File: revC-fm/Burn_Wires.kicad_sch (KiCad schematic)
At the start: 16 parts, among them J6 T1M-04-F-SV-L, K1 PE014006, Q29 MMDT5551-7-F, Q38 BSZ180P03NS3GATMA1, Q39 MMBT2222LT1G, Q41 BSZ180P03NS3GATMA1

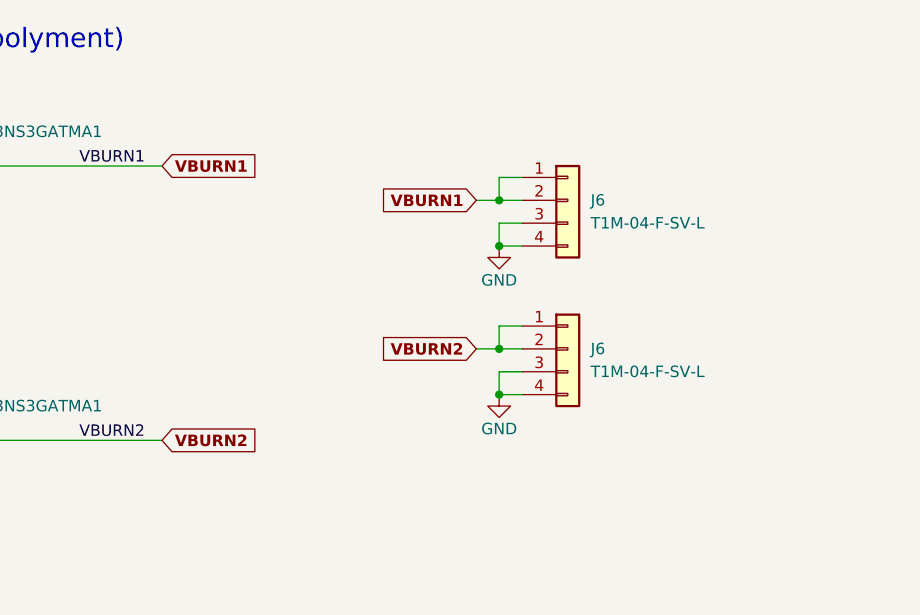
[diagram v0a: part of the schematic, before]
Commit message: routing fm
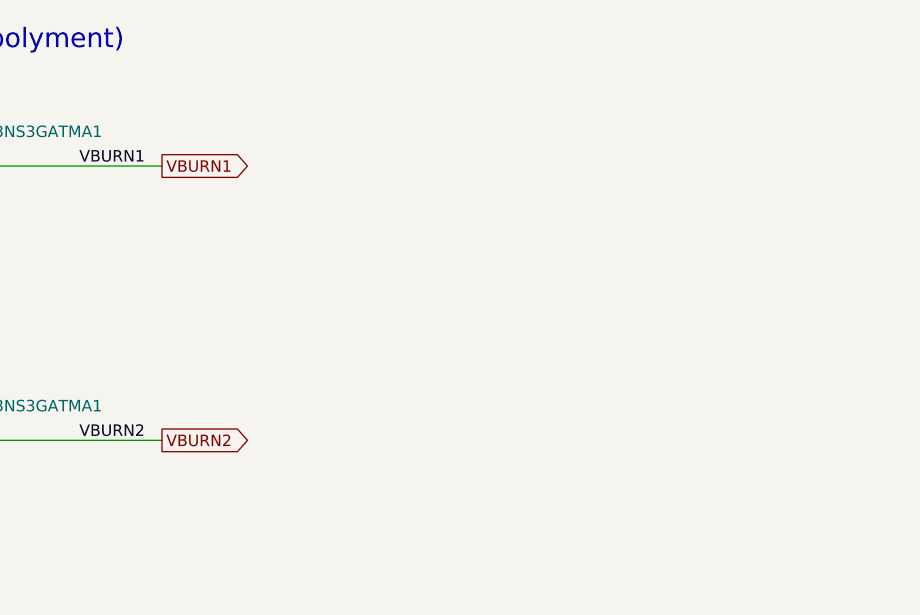
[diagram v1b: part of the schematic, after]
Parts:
- removed J6 (x2): T1M-04-F-SV-L, SierraLobo:SAMTEC_T1M-04-F-SV-L, symbol Connector_Generic:Conn_01x04
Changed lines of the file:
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@@
     (company "Sierra Lobo INC.")
   )
-  (junction (at 252.73 39.37) (diameter 0) (color 0 0 0 0)
-  )
   (junction (at 124.46 30.48) (diameter 0) (color 0 0 0 0)
   )
@@
   (junction (at 58.42 38.1) (diameter 0) (color 0 0 0 0)
   )
-  (junction (at 252.73 50.8) (diameter 0) (color 0 0 0 0)
-  )
   (junction (at 58.42 30.48) (diameter 0) (color 0 0 0 0)
   )
@@
   (junction (at 170.18 60.96) (diameter 0) (color 0 0 0 0)
   )
-  (junction (at 252.73 34.29) (diameter 0) (color 0 0 0 0)
-  )
-  (junction (at 252.73 55.88) (diameter 0) (color 0 0 0 0)
-  )
-  (wire (pts (xy 252.73 36.83) (xy 255.27 36.83))
-    (stroke (width 0) (type default))
-  )
   (wire (pts (xy 170.18 30.48) (xy 170.18 31.75))
     (stroke (width 0) (type default))
@@
     (stroke (width 0) (type default))
   )
-  (wire (pts (xy 252.73 50.8) (xy 255.27 50.8))
-    (stroke (width 0) (type default))
-  )
   (wire (pts (xy 144.78 48.26) (xy 154.94 48.26))
     (stroke (width 0) (type default))
@@
     (stroke (width 0) (type default))
   )
-  (wire (pts (xy 252.73 53.34) (xy 255.27 53.34))
-    (stroke (width 0) (type default))
-  )
   (wire (pts (xy 170.18 60.96) (xy 185.42 60.96))
     (stroke (width 0) (type default))
@@
     (stroke (width 0) (type default))
   )
-  (wire (pts (xy 255.27 31.75) (xy 252.73 31.75))
-    (stroke (width 0) (type default))
-  )
   (wire (pts (xy 170.18 69.85) (xy 170.18 73.025))
     (stroke (width 0) (type default))
@@
     (stroke (width 0) (type default))
   )
-  (wire (pts (xy 252.73 55.88) (xy 252.73 53.34))
-    (stroke (width 0) (type default))
-  )
-  (wire (pts (xy 252.73 31.75) (xy 252.73 34.29))
-    (stroke (width 0) (type default))
-  )
-  (wire (pts (xy 252.73 34.29) (xy 255.27 34.29))
-    (stroke (width 0) (type default))
-  )
   (wire (pts (xy 58.42 52.705) (xy 58.42 55.88))
     (stroke (width 0) (type default))
@@
     (stroke (width 0) (type default))
   )
-  (wire (pts (xy 252.73 39.37) (xy 252.73 36.83))
-    (stroke (width 0) (type default))
-  )
   (wire (pts (xy 124.46 30.48) (xy 170.18 30.48))
     (stroke (width 0) (type default))
   )
-  (wire (pts (xy 250.19 34.29) (xy 252.73 34.29))
-    (stroke (width 0) (type default))
-  )
   (wire (pts (xy 195.58 60.96) (xy 215.265 60.96))
     (stroke (width 0) (type default))
@@
     (stroke (width 0) (type default))
   )
-  (wire (pts (xy 255.27 39.37) (xy 252.73 39.37))
-    (stroke (width 0) (type default))
-  )
   (wire (pts (xy 124.46 60.96) (xy 170.18 60.96))
     (stroke (width 0) (type default))
@@
     (stroke (width 0) (type default))
   )
-  (wire (pts (xy 252.73 48.26) (xy 252.73 50.8))
-    (stroke (width 0) (type default))
-  )
   (wire (pts (xy 38.1 47.625) (xy 41.91 47.625))
     (stroke (width 0) (type default))
@@
     (stroke (width 0) (type default))
   )
-  (wire (pts (xy 250.19 50.8) (xy 252.73 50.8))
-    (stroke (width 0) (type default))
-  )
   (polyline (pts (xy 176.53 162.56) (xy 284.48 162.56))
     (stroke (width 0) (type default))
@@
     (stroke (width 0) (type default))
   )
-  (wire (pts (xy 255.27 48.26) (xy 252.73 48.26))
-    (stroke (width 0) (type default))
-  )
   (wire (pts (xy 58.42 38.1) (xy 63.5 38.1))
     (stroke (width 0) (type default))
   )
   (wire (pts (xy 49.53 47.625) (xy 50.8 47.625))
-    (stroke (width 0) (type default))
-  )
-  (wire (pts (xy 255.27 55.88) (xy 252.73 55.88))
     (stroke (width 0) (type default))
   )
@@
     )
   )
-  (global_label "VBURN1" (shape input) (at 215.265 30.48 0) (fields_autoplaced)
-    (effects (font (size 1.27 1.27) (thickness 0.254) bold) (justify left))
-    (property "Intersheetrefs" "${INTERSHEET_REFS}" (at 1.905 -5.08 0)
-      (effects (font (size 1.27 1.27)) hide)
+  (global_label "VBURN1" (shape output) (at 215.265 30.48 0) (fields_autoplaced)
+    (effects (font (size 1.27 1.27)) (justify left))
+    (property "Intersheetrefs" "${INTERSHEET_REFS}" (at 225.0157 30.48 0)
+      (effects (font (size 1.27 1.27)) (justify left) hide)
     )
   )
@@
     )
   )
-  (global_label "VBURN2" (shape input) (at 250.19 50.8 180) (fields_autoplaced)
-    (effects (font (size 1.27 1.27) (thickness 0.254) bold) (justify right))
-    (property "Intersheetrefs" "${INTERSHEET_REFS}" (at 463.55 -8.89 0)
-      (effects (font (size 1.27 1.27)) (justify left) hide)
-    )
-  )
-  (global_label "VBURN2" (shape input) (at 215.265 60.96 0) (fields_autoplaced)
-    (effects (font (size 1.27 1.27) (thickness 0.254) bold) (justify left))
-    (property "Intersheetrefs" "${INTERSHEET_REFS}" (at 1.905 1.27 0)
-      (effects (font (size 1.27 1.27)) hide)
-    )
-  )
-  (global_label "VBURN1" (shape input) (at 250.19 34.29 180) (fields_autoplaced)
-    (effects (font (size 1.27 1.27) (thickness 0.254) bold) (justify right))
-    (property "Intersheetrefs" "${INTERSHEET_REFS}" (at 463.55 -1.27 0)
+  (global_label "VBURN2" (shape output) (at 215.265 60.96 0) (fields_autoplaced)
+    (effects (font (size 1.27 1.27)) (justify left))
+    (property "Intersheetrefs" "${INTERSHEET_REFS}" (at 225.0157 60.96 0)
       (effects (font (size 1.27 1.27)) (justify left) hide)
     )
@@
     )
   )
-  (symbol (lib_id "power:GND") (at 252.73 39.37 0) (unit 1)
-    (in_bom yes) (on_board yes) (dnp no)
-    (property "Reference" "#PWR0122" (at 252.73 45.72 0)
-      (effects (font (size 1.27 1.27)) hide)
-    )
-    (property "Value" "GND" (at 252.73 43.18 0)
-      (effects (font (size 1.27 1.27)))
-    )
-    (property "Footprint" "" (at 252.73 39.37 0)
-      (effects (font (size 1.27 1.27)) hide)
-    )
-    (property "Datasheet" "" (at 252.73 39.37 0)
-      (effects (font (size 1.27 1.27)) hide)
-    )
-    (pin "1")
-    (instances
-      (project "mainboard"
-        (path "/d1441985-7b63-4bf8-a06d-c70da2e3b78b/00000000-0000-0000-0000-00005cec6476"
-          (reference "#PWR0122") (unit 1)
-        )
-      )
-    )
-  )
   (symbol (lib_id "Transistor_BJT:MMDT5551") (at 167.64 81.28 0) (unit 2)
     (in_bom yes) (on_board yes) (dnp no)
@@
     )
   )
-  (symbol (lib_id "power:GND") (at 252.73 55.88 0) (unit 1)
-    (in_bom yes) (on_board yes) (dnp no)
-    (property "Reference" "#PWR0125" (at 252.73 62.23 0)
-      (effects (font (size 1.27 1.27)) hide)
-    )
-    (property "Value" "GND" (at 252.73 59.69 0)
-      (effects (font (size 1.27 1.27)))
-    )
-    (property "Footprint" "" (at 252.73 55.88 0)
-      (effects (font (size 1.27 1.27)) hide)
-    )
-    (property "Datasheet" "" (at 252.73 55.88 0)
-      (effects (font (size 1.27 1.27)) hide)
-    )
-    (pin "1")
-    (instances
-      (project "mainboard"
-        (path "/d1441985-7b63-4bf8-a06d-c70da2e3b78b/00000000-0000-0000-0000-00005cec6476"
-          (reference "#PWR0125") (unit 1)
-        )
-      )
-    )
-  )
   (symbol (lib_id "Transistor_BJT:MMDT5551") (at 167.64 48.26 0) (unit 2)
     (in_bom yes) (on_board yes) (dnp no)
@@
         )
       )
-    )
-  )
-  (symbol (lib_id "Connector_Generic:Conn_01x04") (at 260.35 50.8 0) (unit 1)
-    (in_bom yes) (on_board yes) (dnp no) (fields_autoplaced)
-    (property "Reference" "J6" (at 262.89 50.7999 0)
-      (effects (font (size 1.27 1.27)) (justify left))
-    )
-    (property "Value" "T1M-04-F-SV-L" (at 262.89 53.3399 0)
-      (effects (font (size 1.27 1.27)) (justify left))
-    )
-    (property "Footprint" "SierraLobo:SAMTEC_T1M-04-F-SV-L" (at 260.35 50.8 0)
-      (effects (font (size 1.27 1.27)) hide)
-    )
-    (property "Datasheet" "~" (at 260.35 50.8 0)
-      (effects (font (size 1.27 1.27)) hide)
-    )
-    (pin "1")
-    (pin "2")
-    (pin "3")
-    (pin "4")
-    (instances
-      (project "mainboard"
-        (path "/d1441985-7b63-4bf8-a06d-c70da2e3b78b/00000000-0000-0000-0000-00005cec60eb"
-          (reference "J6") (unit 1)
-        )
-        (path "/d1441985-7b63-4bf8-a06d-c70da2e3b78b/00000000-0000-0000-0000-00005cec6476"
-          (reference "J5") (unit 1)
-        )
-      )
-    )
-  )
-  (symbol (lib_id "Connector_Generic:Conn_01x04") (at 260.35 34.29 0) (unit 1)
-    (in_bom yes) (on_board yes) (dnp no) (fields_autoplaced)
-    (property "Reference" "J6" (at 262.89 34.2899 0)
-      (effects (font (size 1.27 1.27)) (justify left))
-    )
-    (property "Value" "T1M-04-F-SV-L" (at 262.89 36.8299 0)
-      (effects (font (size 1.27 1.27)) (justify left))
-    )
-    (property "Footprint" "SierraLobo:SAMTEC_T1M-04-F-SV-L" (at 260.35 34.29 0)
-      (effects (font (size 1.27 1.27)) hide)
-    )
-    (property "Datasheet" "~" (at 260.35 34.29 0)
-      (effects (font (size 1.27 1.27)) hide)
-    )
-    (pin "1")
-    (pin "2")
-    (pin "3")
-    (pin "4")
-    (instances
-      (project "mainboard"
-        (path "/d1441985-7b63-4bf8-a06d-c70da2e3b78b/00000000-0000-0000-0000-00005cec60eb"
-          (reference "J6") (unit 1)
-        )
-        (path "/d1441985-7b63-4bf8-a06d-c70da2e3b78b/00000000-0000-0000-0000-00005cec6476"
-          (reference "J4") (unit 1)
-        )
-      )
